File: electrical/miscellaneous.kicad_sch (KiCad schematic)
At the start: 1 part

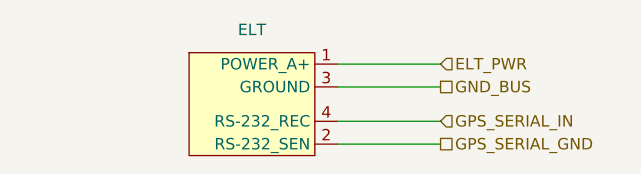
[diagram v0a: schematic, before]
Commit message: Interim check-in
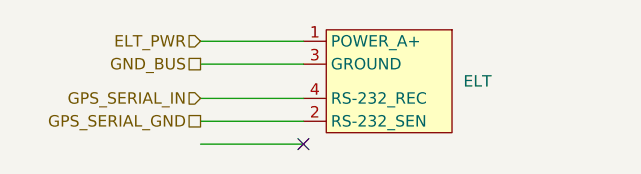
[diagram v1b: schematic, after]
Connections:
- no-connect marks 0 -> 1
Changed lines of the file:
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@@
 		(company "N877RV")
+	)
+	(no_connect
+		(at 132.08 92.71)
 	)
 	(wire
 		(pts
-			(xy 135.89 92.71) (xy 147.32 92.71)
+			(xy 132.08 87.63) (xy 120.65 87.63)
 		)
 		(stroke
@@
 	(wire
 		(pts
-			(xy 135.89 86.36) (xy 147.32 86.36)
+			(xy 132.08 92.71) (xy 120.65 92.71)
+		)
+		(stroke
+			(width 0)
+			(type dash)
+		)
+	)
+	(wire
+		(pts
+			(xy 132.08 83.82) (xy 120.65 83.82)
 		)
 		(stroke
@@
 	(wire
 		(pts
-			(xy 135.89 83.82) (xy 147.32 83.82)
+			(xy 132.08 81.28) (xy 120.65 81.28)
 		)
 		(stroke
@@
 	(wire
 		(pts
-			(xy 135.89 90.17) (xy 147.32 90.17)
+			(xy 132.08 90.17) (xy 120.65 90.17)
 		)
 		(stroke
@@
 		)
 	)
-	(hierarchical_label "GPS_SERIAL_GND"
-		(shape passive)
-		(at 147.32 92.71 0)
+	(hierarchical_label "ELT_PWR"
+		(shape input)
+		(at 120.65 81.28 180)
 		(effects
 			(font
 				(size 1.27 1.27)
 			)
-			(justify left)
+			(justify right)
+		)
+	)
+	(hierarchical_label "GPS_SERIAL_GND"
+		(shape passive)
+		(at 120.65 90.17 180)
+		(effects
+			(font
+				(size 1.27 1.27)
+			)
+			(justify right)
 		)
 	)
 	(hierarchical_label "GND_BUS"
 		(shape passive)
-		(at 147.32 86.36 0)
+		(at 120.65 83.82 180)
 		(effects
 			(font
 				(size 1.27 1.27)
 			)
-			(justify left)
+			(justify right)
 		)
 	)
 	(hierarchical_label "GPS_SERIAL_IN"
 		(shape input)
-		(at 147.32 90.17 0)
+		(at 120.65 87.63 180)
 		(effects
 			(font
 				(size 1.27 1.27)
 			)
-			(justify left)
-		)
-	)
-	(hierarchical_label "ELT_PWR"
-		(shape input)
-		(at 147.32 83.82 0)
-		(effects
-			(font
-				(size 1.27 1.27)
-			)
-			(justify left)
+			(justify right)
 		)
 	)
 	(symbol
 		(lib_id "flyerx:ACK_E-04")
-		(at 119.38 82.55 0)
+		(at 148.59 80.01 0)
+		(mirror y)
 		(unit 1)
 		(exclude_from_sim no)
@@
 		(fields_autoplaced yes)
 		(property "Reference" "ELT"
-			(at 126.365 80.01 0)
+			(at 149.86 85.7249 0)
 			(effects
 				(font
 					(size 1.27 1.27)
 				)
+				(justify right)
 			)
 		)
 		(property "Value" "~"
-			(at 119.38 81.28 0)
+			(at 148.59 78.74 0)
 			(effects
 				(font
 					(size 1.27 1.27)
 				)
+				(hide yes)
 			)
 		)
 		(property "Footprint" ""
-			(at 119.38 81.28 0)
+			(at 148.59 78.74 0)
 			(effects
 				(font
@@
 		)
 		(property "Datasheet" ""
-			(at 119.38 81.28 0)
+			(at 148.59 78.74 0)
 			(effects
 				(font
@@
 		)
 		(property "Description" ""
-			(at 119.38 82.55 0)
+			(at 148.59 80.01 0)
 			(effects
 				(font
